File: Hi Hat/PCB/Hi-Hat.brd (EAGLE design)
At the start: 100 x 50 mm, 92 parts, among them IC1 LM741P, IC2 LM741P, IC3 LM741P, IC4 LM741P, IC5 LM741P, IC6 LM741P, IC7 LM741P, Q1 2N2222A, Q6 2N3904, Q7 2N3904

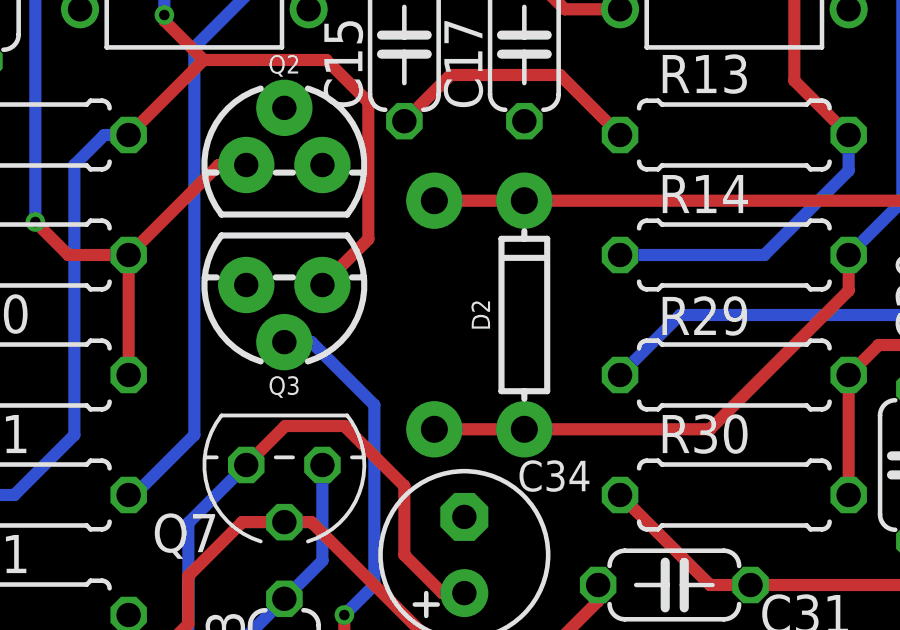
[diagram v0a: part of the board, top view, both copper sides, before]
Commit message: Generated Gerbers
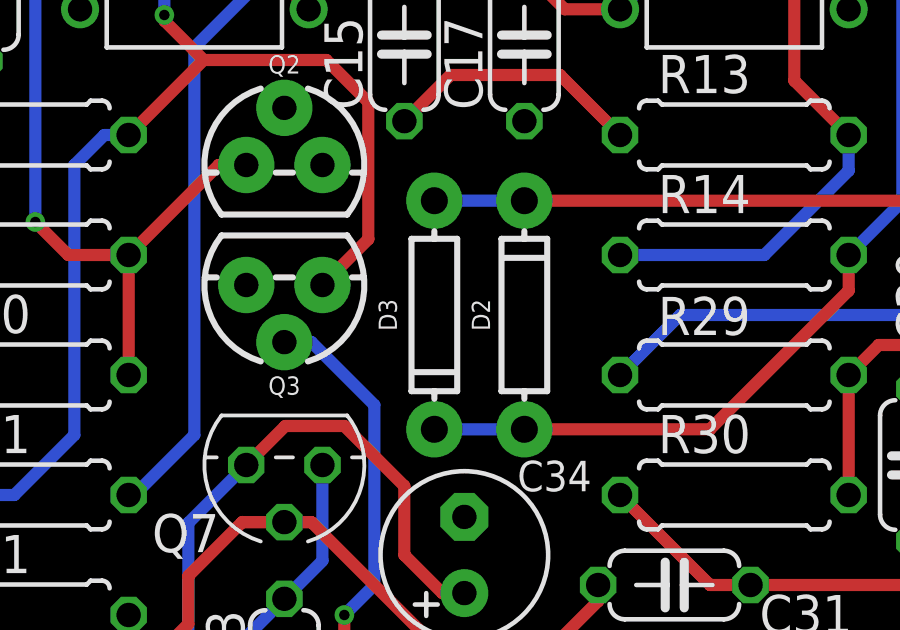
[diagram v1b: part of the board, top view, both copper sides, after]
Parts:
- flipped D3 to the top
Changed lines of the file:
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@@
 <?xml version="1.0" encoding="utf-8"?>
 <!DOCTYPE eagle SYSTEM "eagle.dtd">
-<eagle version="9.3.0">
+<eagle version="9.2.2">
 <drawing>
 <settings>
@@
 <attribute name="VALUE" x="41.143" y="28" size="0.6096" layer="27" font="vector" ratio="20" rot="R90" align="top-center"/>
 </element>
-<element name="D3" library="SparkFun-DiscreteSemi" package="DIODE-1N4148" value="200mA/100V/1V" x="37" y="28" smashed="yes" rot="MR270">
-<attribute name="NAME" x="35.857" y="28" size="0.6096" layer="26" font="vector" ratio="20" rot="MR270" align="bottom-center"/>
-<attribute name="PROD_ID" value="DIO-08378" x="37" y="28" size="1.778" layer="28" rot="MR270" display="off"/>
-<attribute name="VALUE" x="38.143" y="28" size="0.6096" layer="28" font="vector" ratio="20" rot="MR270" align="top-center"/>
+<element name="D3" library="SparkFun-DiscreteSemi" package="DIODE-1N4148" value="200mA/100V/1V" x="37" y="28" smashed="yes" rot="R270">
+<attribute name="NAME" x="35.143" y="28" size="0.6096" layer="25" font="vector" ratio="20" rot="R270" align="bottom-center"/>
+<attribute name="PROD_ID" value="DIO-08378" x="37" y="28" size="1.778" layer="27" rot="R270" display="off"/>
+<attribute name="VALUE" x="35.857" y="28" size="0.6096" layer="27" font="vector" ratio="20" rot="R270" align="top-center"/>
 </element>
 <element name="D5" library="SparkFun-DiscreteSemi" package="DIODE-1N4148" value="200mA/100V/1V" x="81" y="17" smashed="yes" rot="R270">
@@
 <contactref element="D2" pad="A"/>
 <contactref element="D3" pad="C"/>
-<wire x1="40" y1="24.19" x2="37" y2="24.19" width="0.4064" layer="1"/>
+<wire x1="40" y1="24.19" x2="37" y2="24.19" width="0.4064" layer="16"/>
 <wire x1="40" y1="24.19" x2="46.19" y2="24.19" width="0.4064" layer="1"/>
 <wire x1="50.81" y1="28.81" x2="50.81" y2="30" width="0.4064" layer="1"/>
@@
 <contactref element="D3" pad="A"/>
 <contactref element="R22" pad="1"/>
-<wire x1="37" y1="31.81" x2="40" y2="31.81" width="0.4064" layer="1"/>
+<wire x1="37" y1="31.81" x2="40" y2="31.81" width="0.4064" layer="16"/>
 <wire x1="40" y1="31.81" x2="63.81" y2="31.81" width="0.4064" layer="1"/>
 <wire x1="63.81" y1="31.81" x2="66" y2="34" width="0.4064" layer="1"/>
